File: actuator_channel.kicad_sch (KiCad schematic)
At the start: 1 part

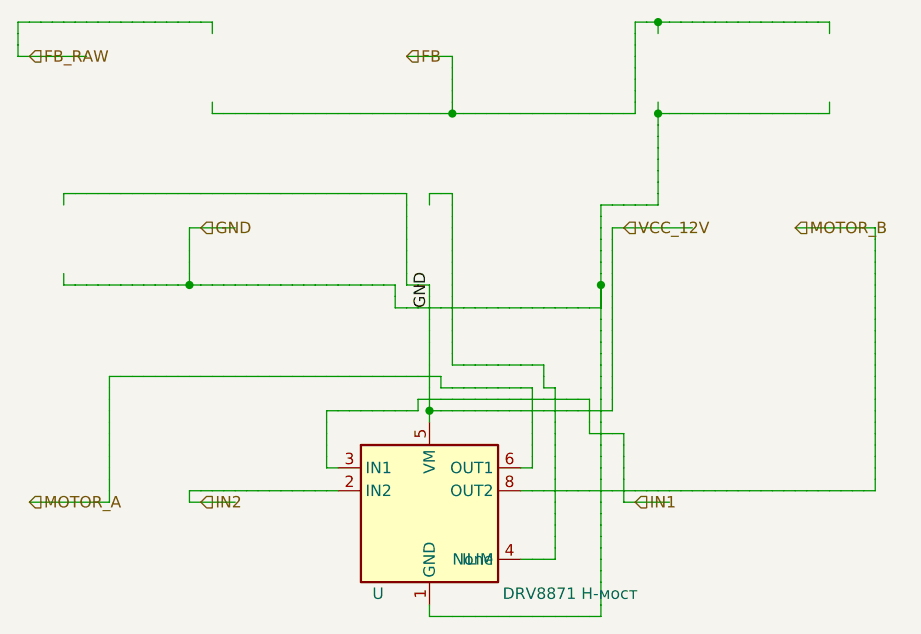
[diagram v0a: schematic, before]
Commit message: fix writer
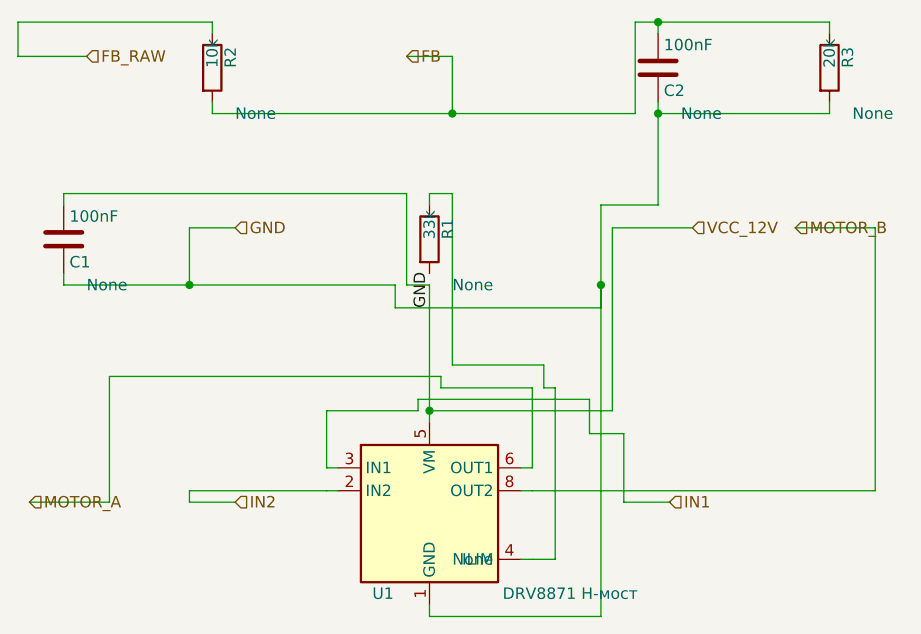
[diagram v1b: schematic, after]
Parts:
- removed U: DRV8871 H-мост, symbol Driver_Motor:DRV8871DDA
- added C1, C2: 100nF, symbol Device:C
- added R1: 33k, symbol Device:R
- added R2: 10k, symbol Device:R
- added R3: 20k, symbol Device:R
- added U1: DRV8871 H-мост, symbol Driver_Motor:DRV8871DDA
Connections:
- net FB: now also C2.1, R2.2, R3.1
- net FB_RAW: now also R2.1
- net GND: now also C1.1, C1.2, C2.2, R3.2, U1.1 (GND), U1.5 (VM), U1.7 (GND), U1.9 (GND)
- net IN2: now also U1.2 (IN2)
- new net: R1.1, U1.4 (ILIM)
- new net IN1: U1.3 (IN1)
- new net MOTOR_A: U1.6 (OUT1)
- new net MOTOR_B: U1.8 (OUT2)
